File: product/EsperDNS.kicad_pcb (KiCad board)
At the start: 2 copper layers, 45.1 x 83.7 mm, 57 parts, among them J1 10118192-0001LF, J2 ARJM11A3, J3 Conn_02x05_Odd_Even, Q1 Q_NMOS_GSD, Q2 Q_NMOS_GSD, Q3 Q_NMOS_GSD, SW1 SW_SPST, SW2 SW_SPST, U1 AZ1117-3.3, U2 LAN8720A, U3 ESP32-WROOM-32D

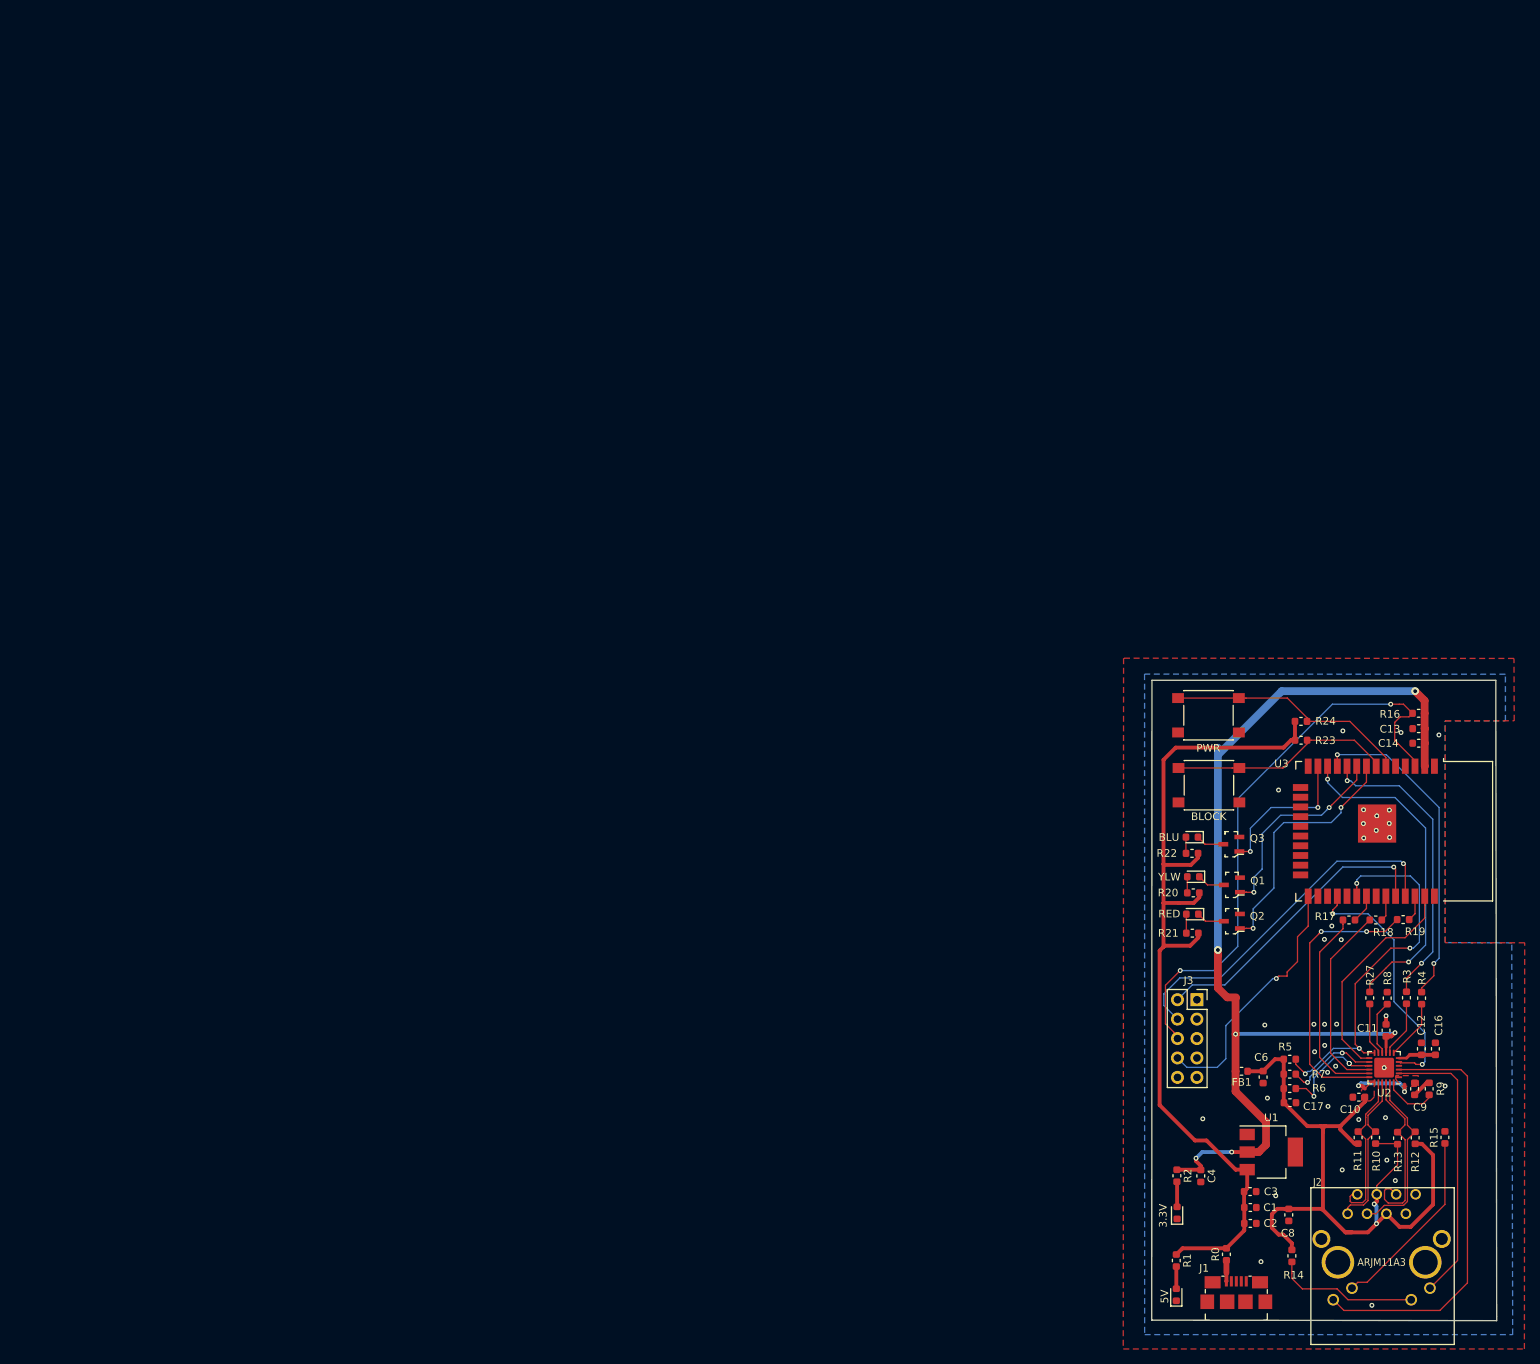
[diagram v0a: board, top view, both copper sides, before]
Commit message: Finished layout
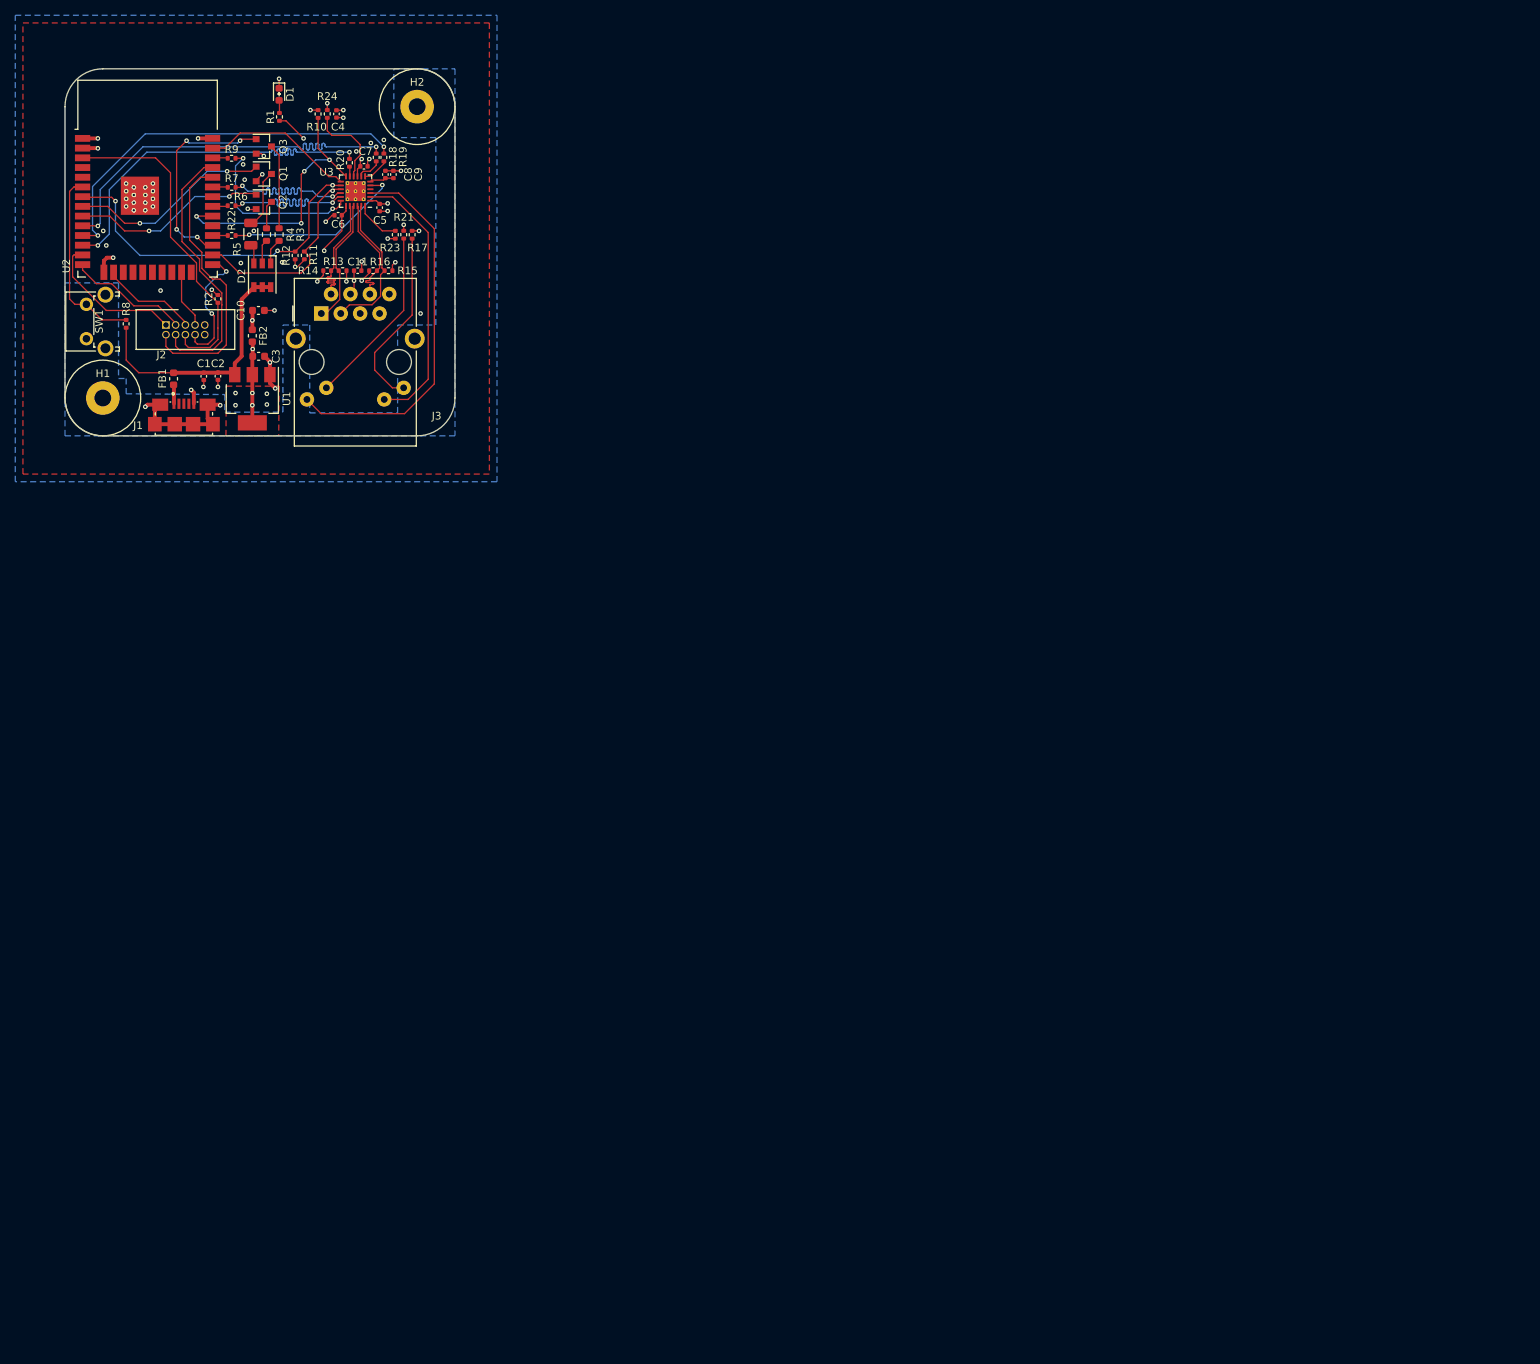
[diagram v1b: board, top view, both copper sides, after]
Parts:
- removed C12: 0.1uF, Capacitor_SMD:C_0603_1608Metric
- removed C13: 10uF, Capacitor_SMD:C_0603_1608Metric
- removed C14, C16, C17: 1uF, Capacitor_SMD:C_0603_1608Metric
- removed D3: YLW, Diode_SMD:D_0603_1608Metric
- removed D4: RED, Diode_SMD:D_0603_1608Metric
- removed D5: BLUE, Diode_SMD:D_0603_1608Metric
- removed R0: 0, Resistor_SMD:R_0603_1608Metric
- removed R27: 100, Resistor_SMD:R_0603_1608Metric
- removed SW2: SW_SPST, Button_Switch_SMD:SW_Push_1P1T_NO_6x6mm_H9.5mm
- added C5: 0.1uF, Capacitor_SMD:C_0402_1005Metric, F.Cu at (15.7, -5.85)
- added C7: 0.1uF, Capacitor_SMD:C_0402_1005Metric, F.Cu at (13.6, -11.2)
- added FB2: Ferrite_Bead, Inductor_SMD:L_0603_1608Metric, F.Cu at (-1.00, 10.9)
- added H1: MountingHole, MountingHole:MountingHole_2.2mm_M2_Pad, F.Cu at (-20.6, 19.1)
- added H2: MountingHole, MountingHole:MountingHole_2.2mm_M2_Pad, F.Cu at (20.6, -19.1)
- C1: value 10uF -> 1uF; footprint Capacitor_SMD:C_0603_1608Metric -> Capacitor_SMD:C_0402_1005Metric
- C10: value 0.1uF -> 10uF
- C11, C2, C8: footprint Capacitor_SMD:C_0603_1608Metric -> Capacitor_SMD:C_0402_1005Metric
- C3: value 1uF -> 10uF
- C4: value 4.7uF -> 1uF; footprint Capacitor_SMD:C_0603_1608Metric -> Capacitor_SMD:C_0402_1005Metric
- C6: value 4.7uF -> 0.1uF; footprint Capacitor_SMD:C_0603_1608Metric -> Capacitor_SMD:C_0402_1005Metric
- C9: value 0.1uF -> 1uF; footprint Capacitor_SMD:C_0603_1608Metric -> Capacitor_SMD:C_0402_1005Metric
- D2: value GRN -> RS-3535MWAP; footprint Diode_SMD:D_0603_1608Metric -> LED_SMD:LED_RGB_PLCC-6
- J1: footprint digikey-footprints:USB_Micro_B_Female_10118192 -> Esper_Footprints:AMPHENOL_10118192-0001LF
- J2: value ARJM11A3 -> Conn_02x05_Odd_Even; footprint My Footprints:ARJM11A3-009-AB-ER2-T -> Esper_Footprints:CNC_3220-10-0100-00
- J3: value Conn_02x05_Odd_Even -> RJ45_Amphenol_RJMG1BD3B8K1ANR; footprint Connector_PinSocket_2.54mm:PinSocket_2x05_P2.54mm_Vertical -> Connector_RJ:RJ45_Amphenol_RJMG1BD3B8K1ANR
- Q1, Q2, Q3: footprint digikey-footprints:SOT-23-3 -> Package_TO_SOT_SMD:SOT-23
- R1, R13, R24, R8: footprint Resistor_SMD:R_0603_1608Metric -> Resistor_SMD:R_0402_1005Metric
- R10, R11, R12: value 49.9 -> 10K; footprint Resistor_SMD:R_0603_1608Metric -> Resistor_SMD:R_0402_1005Metric
- R14, R15: value 270 -> 49.9; footprint Resistor_SMD:R_0603_1608Metric -> Resistor_SMD:R_0402_1005Metric
- R16, R6, R7: value 10K -> 49.9; footprint Resistor_SMD:R_0603_1608Metric -> Resistor_SMD:R_0402_1005Metric
- R17: value 100 -> 270; footprint Resistor_SMD:R_0603_1608Metric -> Resistor_SMD:R_0402_1005Metric
- R18, R19: value 100 -> 49.9; footprint Resistor_SMD:R_0603_1608Metric -> Resistor_SMD:R_0402_1005Metric
- R2: value 470 -> 10K; footprint Resistor_SMD:R_0603_1608Metric -> Resistor_SMD:R_0402_1005Metric
- R20, R22: value 470 -> 49.9; footprint Resistor_SMD:R_0603_1608Metric -> Resistor_SMD:R_0402_1005Metric
- R21: value 470 -> 270; footprint Resistor_SMD:R_0603_1608Metric -> Resistor_SMD:R_0402_1005Metric
- R23: value 10K -> 12.1K; footprint Resistor_SMD:R_0603_1608Metric -> Resistor_SMD:R_0402_1005Metric
- R3, R4: value 100 -> 47
- R5: value 10K -> 82; footprint Resistor_SMD:R_0603_1608Metric -> Resistor_SMD:R_1206_3216Metric
- R9: value 12.1K -> 49.9; footprint Resistor_SMD:R_0603_1608Metric -> Resistor_SMD:R_0402_1005Metric
- SW1: value SW_SPST -> PTS645VH83-2 LFS; footprint Button_Switch_SMD:SW_Push_1P1T_NO_6x6mm_H9.5mm -> Button_Switch_THT:SW_Tactile_SPST_Angled_PTS645Vx83-2LFS
- U1: value AZ1117-3.3 -> AZ1117EH-3.3
- U2: value LAN8720A -> ESP32-WROOM-32D; footprint Package_DFN_QFN:QFN-24-1EP_4x4mm_P0.5mm_EP2.6x2.6mm -> RF_Module:ESP32-WROOM-32
- U3: value ESP32-WROOM-32D -> LAN8720A; footprint RF_Module:ESP32-WROOM-32 -> Package_DFN_QFN:QFN-24-1EP_4x4mm_P0.5mm_EP2.6x2.6mm_ThermalVias
- moved J2 200.8 mm to (-12.3, 9.50), turned to 90 degrees
- moved R9 198.3 mm to (-3.71, -12.3), turned to 0 degrees
- moved U2 197.4 mm to (-14.7, -6.64), turned to 0 degrees
- moved D1 196.0 mm to (2.50, -20.7), turned to 270 degrees
- moved R10 192.5 mm to (7.60, -18.1), turned to 270 degrees
- moved R1 190.1 mm to (2.55, -17.7), turned to 90 degrees
- moved R8 187.0 mm to (-17.5, 9.35)
- moved R12 186.5 mm to (4.60, 0.41)
- moved R4 181.1 mm to (0.85, -2.33)
- moved J1 180.9 mm to (-9.95, 19.8)
- moved R7 180.5 mm to (-3.70, -8.50)
- moved R14 180.3 mm to (8.79, 2.40), turned to 0 degrees
- moved R6 180.2 mm to (-3.71, -6.10)
- moved C8 180.2 mm to (16.4, -10.2), turned to 90 degrees
- moved R11 179.7 mm to (5.80, 0.40)
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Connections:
- C10 pad 1: AVDD -> +3.3VA
- C11 pad 1: +3V3 -> +3.3VA
- C3 pad 1: VBUS -> +3V3
- C4 pad 1: +3V3 -> +3.3VA
- C6 pad 1: AVDD -> +3.3VA
- C8 pad 1: AVDD -> VDDCR
- C9 pad 1: AVDD -> VDDCR
- D2 pad 1: GND -> Net-(D2-Pad1)
- FB1 pad 1: AVDD -> VBUS
- FB1 pad 2: +3V3 -> Net-(FB1-Pad2)
- J1 pad 1: Net-(J1-Pad1) -> Net-(FB1-Pad2)
- J2 pad 1: /Page 1/TD+ -> MTMS
- J2 pad 2: /Page 1/TD- -> TX
- J2 pad 3: /Page 1/RD+ -> MTDI
- J2 pad 4: AVDD -> RX
- J2 pad 5: AVDD -> MTCK
- J2 pad 6: /Page 1/RD- -> EN
- J2 pad 7: Net-(J2-Pad7) -> MTDO
- J2 pad 8: GND -> IO0
- Q1 pad 1: YELLOW -> Red
- Q1 pad 3: Net-(D3-Pad1) -> Net-(Q1-Pad3)
- Q2 pad 1: RED -> Green
- Q2 pad 3: Net-(D4-Pad1) -> Net-(Q2-Pad3)
- Q3 pad 1: BLUE -> Blue
- Q3 pad 3: Net-(D5-Pad1) -> Net-(Q3-Pad3)
- R1 pad 1: VBUS -> +3V3
- R10 pad 1: AVDD -> +3.3VA
- R10 pad 2: /Page 1/TD+ -> MDIO
- R11 pad 1: AVDD -> +3.3VA
- R11 pad 2: /Page 1/TD- -> nRST
- R12 pad 1: AVDD -> +3.3VA
- R12 pad 2: /Page 1/RD+ -> nINT
- R13 pad 1: AVDD -> +3.3VA
- R13 pad 2: /Page 1/RD- -> /Ethernet/TD+
- R14 pad 1: AVDD -> +3.3VA
- R14 pad 2: Net-(J2-PadYLWA) -> /Ethernet/TD-
- R15 pad 1: Net-(J2-PadGRNC) -> +3.3VA
- R15 pad 2: GND -> /Ethernet/RD+
- R16 pad 1: EN -> +3.3VA
- R16 pad 2: +3V3 -> /Ethernet/RD-
- R17 pad 1: Net-(R17-Pad1) -> +3.3VA
- R17 pad 2: TXD0 -> /Ethernet/LEDY_A
- R18 pad 1: Net-(R18-Pad1) -> /Ethernet/RX0_R
- R18 pad 2: TXEN -> RXD0
- R19 pad 1: Net-(R19-Pad1) -> /Ethernet/RX1_R
- R19 pad 2: TXD1 -> RXD1
- R2 pad 1: +3V3 -> EN
- R2 pad 2: Net-(D2-Pad2) -> +3V3
- R20 pad 1: VBUS -> /Ethernet/CRS_DV_R
- R20 pad 2: Net-(D3-Pad2) -> CRS_DV
- R21 pad 1: VBUS -> /Ethernet/LEDG_K
- R21 pad 2: Net-(D4-Pad2) -> GND
- R22 pad 1: VBUS -> CLK50MHZ
- R22 pad 2: Net-(D5-Pad2) -> /ESP32/CLK_R
- R23 pad 1: VBUS -> /Ethernet/RBIAS
- R23 pad 2: BLOCK -> GND
- R24 pad 1: VBUS -> /Ethernet/PHYAD0
- R24 pad 2: RESTART -> GND
- R3 pad 1: /Page 1/RX0 -> Net-(D2-Pad1)
- R3 pad 2: RXD0 -> Net-(Q3-Pad3)
- R4 pad 1: /Page 1/RX1 -> Net-(D2-Pad2)
- R4 pad 2: RXD1 -> Net-(Q2-Pad3)
- R5 pad 1: AVDD -> Net-(D2-Pad3)
- R5 pad 2: MDIO -> Net-(Q1-Pad3)
- R6 pad 1: AVDD -> /ESP32/TXD0_R
- R6 pad 2: /Page 1/nRST -> TXD0
- R7 pad 1: AVDD -> /ESP32/TXEN_R
- R7 pad 2: /Page 1/nINT -> TXEN
- R8 pad 1: /Page 1/PHYAD0 -> VBUS
- R8 pad 2: GND -> Block
- R9 pad 1: /Page 1/RBIAS -> /ESP32/TXD1_R
- R9 pad 2: GND -> TXD1
- SW1 pad 2: BLOCK -> Block
- U1 pad 4: (no net) -> +3V3
- U2 pad 1: AVDD -> GND
- U2 pad 10: /Page 1/PHYAD0 -> RXD0
- U2 pad 11: /Page 1/CRS_DV -> RXD1
- U2 pad 12: MDIO -> CRS_DV
- U2 pad 13: MDC -> MTMS
- U2 pad 14: /Page 1/nINT -> MTDI
- U2 pad 15: /Page 1/nRST -> GND
- U2 pad 16: TXEN -> MTCK
- U2 pad 17: TXD0 -> Net-(U2-Pad17)
- U2 pad 18: TXD1 -> Net-(U2-Pad18)
- U2 pad 19: AVDD -> Net-(U2-Pad19)
- U2 pad 2: LED2_nINTSEL -> +3V3
- U2 pad 20: /Page 1/TD- -> Net-(U2-Pad20)
- U2 pad 21: /Page 1/TD+ -> Net-(U2-Pad21)
- U2 pad 22: /Page 1/RD- -> Net-(U2-Pad22)
- U2 pad 23: /Page 1/RD+ -> MTDO
- U2 pad 24: /Page 1/RBIAS -> Net-(U2-Pad24)
- U2 pad 25: GND -> IO0
- U2 pad 3: LED1_REGOFF -> EN
- U2 pad 5: CLK50MHZ -> Net-(U2-Pad5)
- U2 pad 6: VDDCR -> Block
- U2 pad 7: /Page 1/RX1 -> nINT
- U2 pad 8: /Page 1/RX0 -> Red
- U2 pad 9: +3V3 -> Green
- U3 pad 1: GND -> +3.3VA
- U3 pad 10: RXD0 -> /Ethernet/PHYAD0
- U3 pad 11: RXD1 -> /Ethernet/CRS_DV_R
- U3 pad 12: CRS_DV_r -> MDIO
- U3 pad 13: BLUE -> MDC
- U3 pad 14: Net-(U3-Pad14) -> nINT
- U3 pad 15: GND -> nRST
- U3 pad 16: Net-(U3-Pad16) -> TXEN
- U3 pad 17: Net-(U3-Pad17) -> TXD0
- U3 pad 18: Net-(U3-Pad18) -> TXD1
- U3 pad 19: Net-(U3-Pad19) -> +3.3VA
- U3 pad 2: +3V3 -> LED2_nINTSEL
- U3 pad 20: Net-(U3-Pad20) -> /Ethernet/TD-
- U3 pad 21: Net-(U3-Pad21) -> /Ethernet/TD+
- U3 pad 22: Net-(U3-Pad22) -> /Ethernet/RD-
- U3 pad 23: CLKEN -> /Ethernet/RD+
- U3 pad 24: Net-(U3-Pad24) -> /Ethernet/RBIAS
- U3 pad 25: BOOTMODE -> GND
- U3 pad 3: EN -> LED1_REGOFF
- U3 pad 5: Net-(U3-Pad5) -> CLK50MHZ
- U3 pad 6: RESTART -> VDDCR
- U3 pad 7: BLOCK -> /Ethernet/RX1_R
- U3 pad 8: RED -> /Ethernet/RX0_R
- U3 pad 9: YELLOW -> +3V3
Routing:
- net +3V3: track 134.1 -> 20.1 mm, vias 6 -> 12
- net AVDD: track 107.6 -> 0.00 mm, vias 4 -> 0
- net VBUS: track 116.4 -> 36.4 mm
- net CRS_DV: track 0.00 -> 49.9 mm, vias 0 -> 2
- net nINT: track 0.00 -> 45.8 mm, vias 0 -> 3
- net CRS_DV_r: track 43.1 -> 0.00 mm, vias 2 -> 0
- net EN: track 76.8 -> 42.8 mm, vias 2 -> 0
- net BOOTMODE: track 33.9 -> 0.00 mm, vias 1 -> 0
- net RED: track 32.7 -> 0.00 mm, vias 2 -> 0
- net RESTART: track 31.8 -> 0.00 mm
- net BLOCK: track 29.4 -> 0.00 mm
- net GND: track 3.67 -> 32.1 mm, vias 37 -> 49
- net +3.3VA: track 0.00 -> 27.2 mm, vias 0 -> 12
- net Blue: track 0.00 -> 27.1 mm, vias 0 -> 4
- net YELLOW: track 27.0 -> 0.00 mm, vias 2 -> 0
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- added copper zone on Pwr, net +3.3VA
- added copper zone on F.Cu, net +3V3
- added copper zone on Pwr, net +3V3
- added copper zone on B.Cu, net Earth
- added copper zone on Gnd, net GND
- removed copper zone on F.Cu, net AVDD
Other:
- board size 45.1 x 83.7 mm -> 51 x 48 mm
- copper layers 2 -> 4
- net class Default: clearance 0.1524 -> 0.127; trace_width 0.1524 -> 0.127; via_dia 0.635 -> 0.6; via_drill 0.3302 -> 0.3
- rule pad_to_mask_clearance: 0.051 -> 0
- rule trace_clearance: 0.1524 -> 0.127
- rule trace_min: 0.1524 -> 0.127
- rule via_min_drill: 0.3302 -> 0.3
- rule via_min_size: 0.635 -> 0.6
- board text removed: "3.3V"
- board text removed: "5V"
- board text removed: "BLOCK"
- board text removed: "BLU"
- board text removed: "PWR"
- board text removed: "RED"
- board text removed: "YLW"
